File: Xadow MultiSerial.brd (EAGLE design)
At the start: 25.4 x 20.3 mm, 28 parts, among them J1 12p 0.5mm bottom contact, J2 12p 0.5mm bottom contact, J3 12p 0.5mm bottom contact, J4 12p 0.5mm bottom contact, U1 SC16IS752, U2 TXB0106PWR

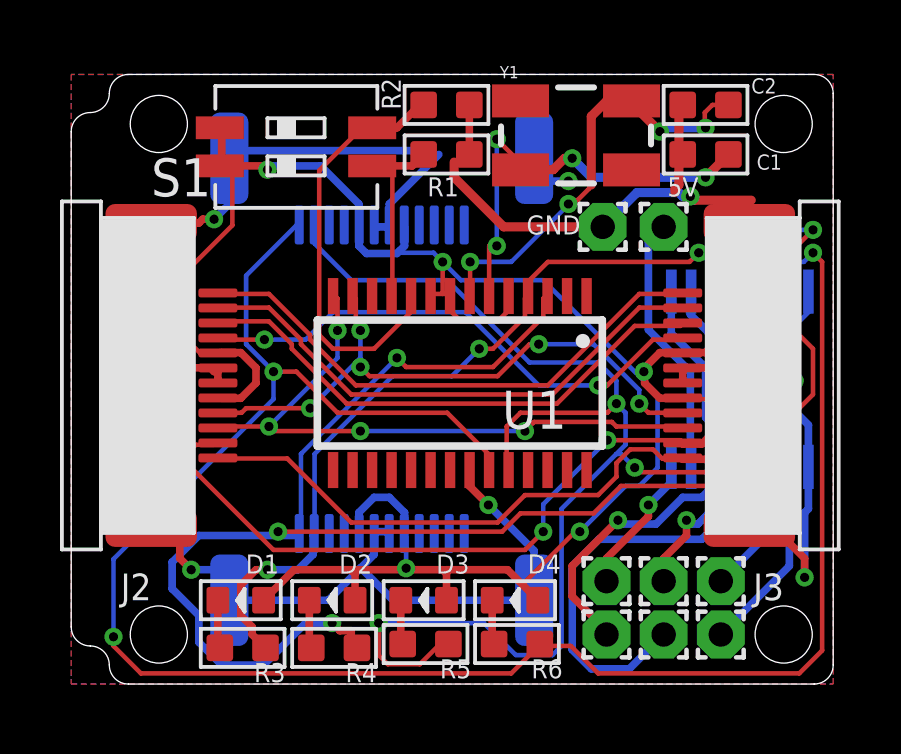
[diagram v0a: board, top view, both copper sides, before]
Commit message: Added mini usb and mosfet based level shifter
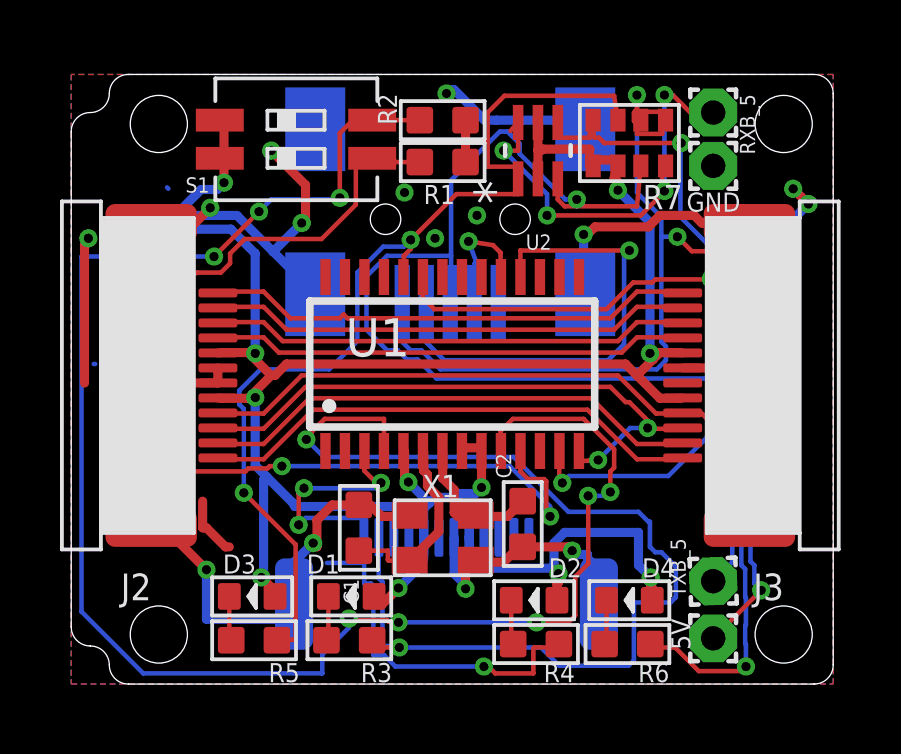
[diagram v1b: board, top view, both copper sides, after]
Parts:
- removed RXA, RXB, RXI, TXA, TXB, TXO: (no value), wirepad:1,6/0,8
- removed Y1: (no value), SparkFun-FreqCtrl:CRYSTAL-SMD-5X3
- added R7: 10K, Discrete:1206-8-3.3X2.4
- added RXB_5, TXB_5: (no value), wirepad:1,6/0,8
- added X1: CTS_32X25_SMD, cts_crystal:CTS_32X25
- J1: value 12p 0.5mm bottom contact -> MINI-USB-5P-3400020P1; device template:12P-0.5 -> OPL Eagle Library:MINI-B-SMD
- U2: value TXB0106PWR -> BSS138PS; device Texas Instruments_By_element14_Batch_1:SOP65P640X120-16N -> NXP_By_element14_Batch_1:SOT65P210X110-6N
- moved C1 17.0 mm to (11.7, 6.22), turned to 270 degrees
- moved C2 15.2 mm to (17.1, 6.35), turned to 90 degrees
- moved 5V 13.8 mm to (23.5, 2.54)
- moved U2 10.2 mm to (17.7, 18.8), flipped to the top, turned to 90 degrees
- moved R4 6.73 mm to (17.6, 2.35)
- moved D2 6.73 mm to (17.5, 3.81)
- moved D3 5.72 mm to (8.13, 3.94)
- moved R5 5.72 mm to (8.19, 2.48)
- moved GND 4.21 mm to (23.5, 18.3)
- moved D4 3.81 mm to (20.7, 3.81)
- moved D1 3.69 mm to (11.4, 3.94)
- moved R6 3.68 mm to (20.6, 2.35)
- moved R3 3.57 mm to (11.4, 2.48)
- moved J1 2.41 mm to (14.7, 17.9)
- moved J4 2.16 mm to (14.6, 3.56)
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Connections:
- removed net N$18: RXI.1, U2.16
- removed net N$19: TXO.1, U2.14
- removed net N$20: RXA.1, U2.13
- removed net N$21: TXA.1, U2.12
- removed net N$22: RXB.1, U2.11
- removed net N$23: TXB.1, U2.10
- removed net N$4: 5V.1, U2.15
- new net 5V: 5V.1, J1.1, R7.1, R7.2
- new net GPIO0: J1.2, U1.18
- new net GPIO1: J1.4, U1.19
- new net RXB_5: R7.8, RXB_5.1, U2.6
- new net TXB_5: J1.3, R7.7, TXB_5.1, U2.3
- net 3V3: now also R7.5, R7.6, U2.5; no longer J1.5, J1.8, U2.8
- net GND: now also J1.5, J1.P$1, J1.P$2, J1.P$3, J1.P$4, X1.2, X1.4; no longer J1.6, J1.7, J1.P1, J1.P2, U2.9
- net N$1: now also X1.1; no longer Y1.1
- net N$2: now also X1.3; no longer Y1.3
- net PD2/RXI/D0: no longer U2.1
- net PD3/TXO/D1: no longer U2.3
- net RXA: no longer U2.4
- net RXB: now also R7.3, U2.1; no longer J1.2, U2.6
- net TXA: no longer U2.5
- net TXB: now also R7.4, U2.4; no longer J1.1, U2.7
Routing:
- net N$5: track 14.1 -> 56.7 mm, vias 0 -> 8
- net 5V: track 0.00 -> 40.3 mm, vias 0 -> 4
- net TXB_5: track 0.00 -> 39.4 mm, vias 0 -> 1
- net TXA: track 57.5 -> 21.0 mm
- net N$3: track 6.22 -> 34.2 mm, vias 0 -> 2
- net TXB: track 66.5 -> 38.8 mm
- net RXB: track 49.7 -> 33.4 mm, vias 4 -> 2
- net GPIO0: track 0.00 -> 16.1 mm, vias 0 -> 1
- net RXB_5: track 0.00 -> 14.9 mm, vias 0 -> 4
- net N$21: track 14.4 -> 0.00 mm
- net GND: track 83.8 -> 72.3 mm, vias 7 -> 17
- net PD2/RXI/D0: track 27.8 -> 16.8 mm, vias 3 -> 0
- net N$2: track 14.7 -> 4.78 mm, vias 4 -> 0
- net RXA: track 26.9 -> 36.5 mm, vias 3 -> 2
- net N$19: track 9.30 -> 0.00 mm, vias 1 -> 0
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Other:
- board text added: "v2.0 26/02/2015"
- board text removed: "v1.0 14/09/2014"
